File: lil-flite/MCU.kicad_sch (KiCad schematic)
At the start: 12 parts, among them SW401 PTS645SM70-2 LFS, SW402 PTS645SM70-2 LFS, U101 STM32F103C8T6, U401 W25Q128JVSIQ

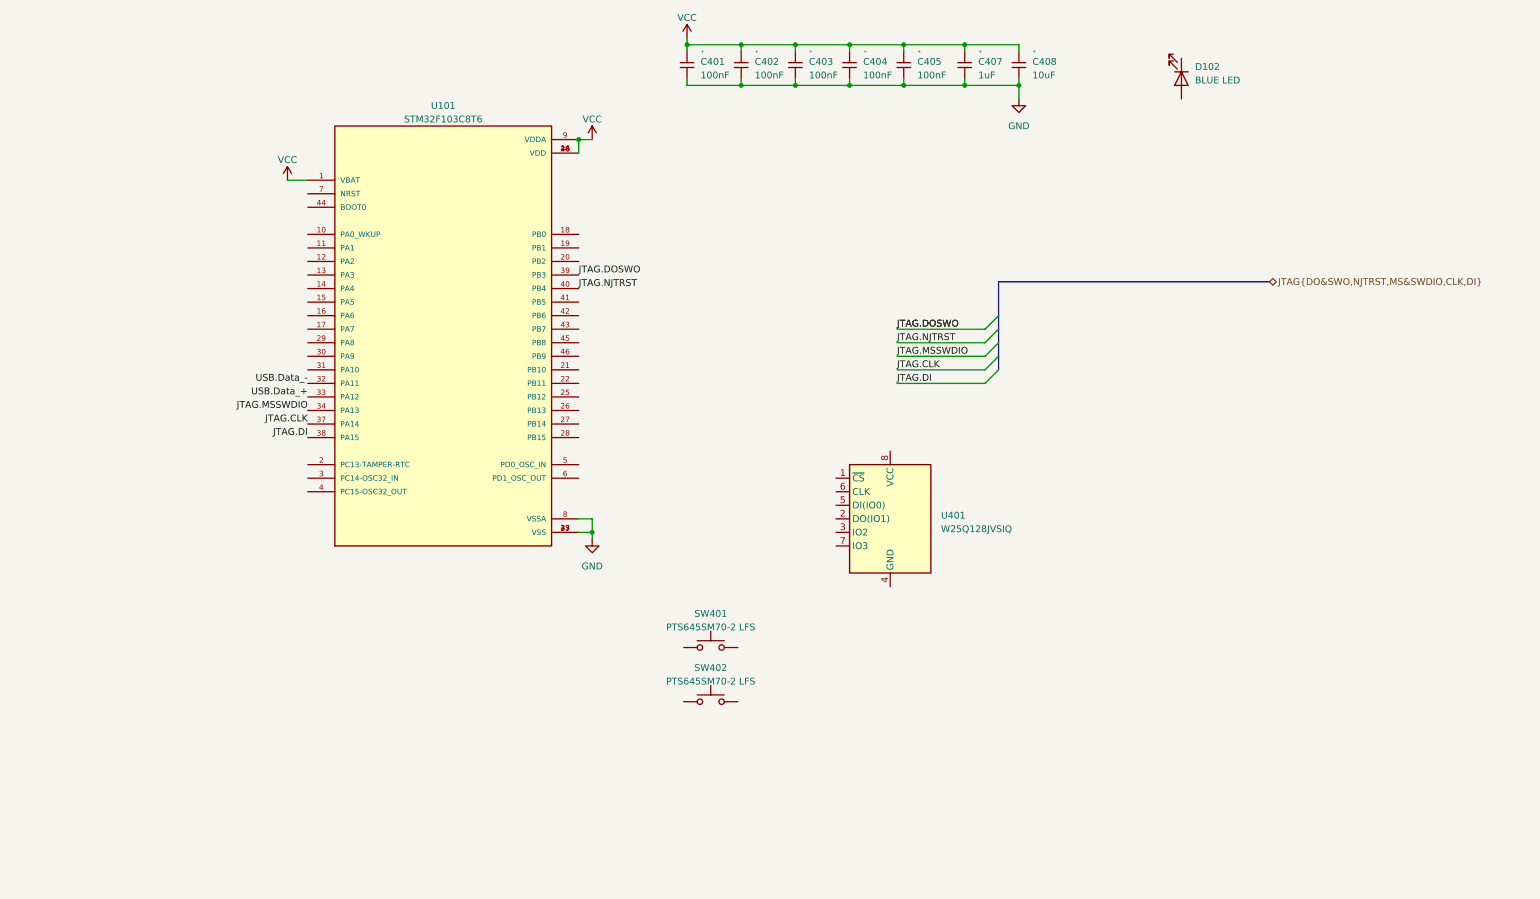
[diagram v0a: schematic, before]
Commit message: Almost finished
Need to double check everything
routing done
more vias maybe
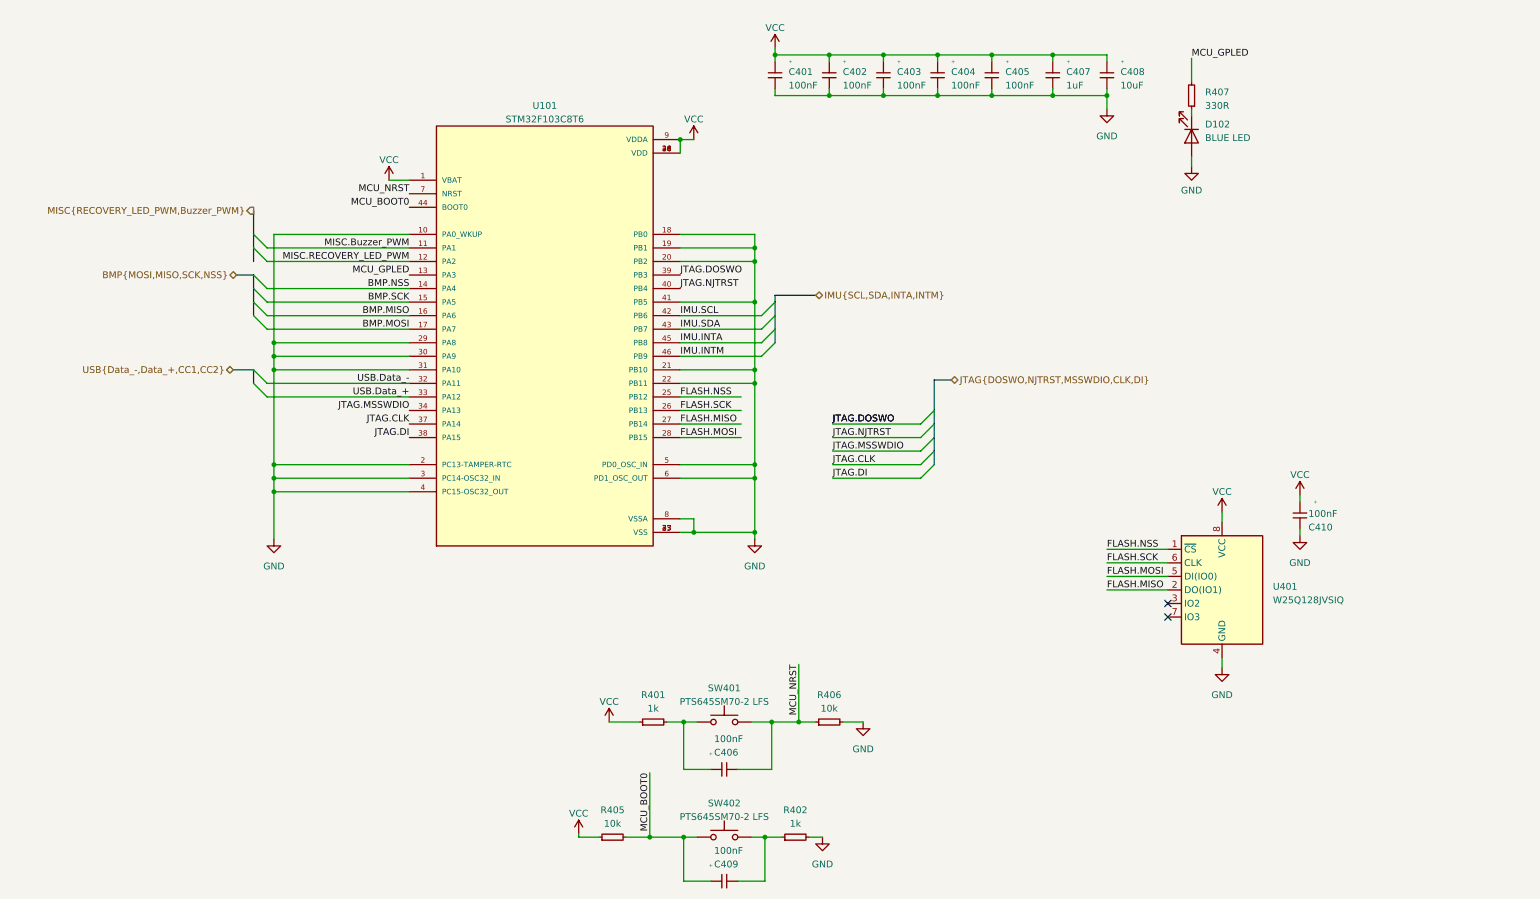
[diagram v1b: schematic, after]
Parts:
- added C406, C409, C410: 100nF, Capacitor_SMD:C_0603_1608Metric_Pad1.08x0.95mm_HandSolder, symbol PCM_Generic-50:C,IEC
- added R401, R402: 1k, Resistor_SMD:R_0603_1608Metric_Pad0.98x0.95mm_HandSolder, symbol PCM_Generic-50:R,IEC
- added R405, R406: 10k, Resistor_SMD:R_0603_1608Metric_Pad0.98x0.95mm_HandSolder, symbol PCM_Generic-50:R,IEC
- added R407: 330R, Resistor_SMD:R_0603_1608Metric_Pad0.98x0.95mm_HandSolder, symbol PCM_Generic-50:R,IEC
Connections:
- net GND: now also D102.2 (A), U101.10 (PA0_WKUP), U101.18 (PB0), U101.19 (PB1), U101.2 (PC13-TAMPER-RTC), U101.20 (PB2), U101.21 (PB10), U101.22 (PB11), U101.29 (PA8), U101.3 (PC14-OSC32_IN), U101.30 (PA9), U101.31 (PA10), U101.4 (PC15-OSC32_OUT), U101.41 (PB5), U101.5 (PD0_OSC_IN), U101.6 (PD1_OSC_OUT), U401.4 (GND), C410.1 (+), R402.2 (-), R406.2 (-)
- net VCC: now also U401.8 (VCC), C410.2 (-), R401.1 (+), R405.1 (+)
- net MCU_BOOT0: now reaches SW402.1, SW402.3
- net MCU_BOOT0: now also U101.44 (BOOT0), C409.2 (-), R405.2 (-)
- net at SW402.2, SW402.4: now also C409.1 (+), R402.1 (+)
- net at D102.1 (K): now also R407.1 (+)
- net at SW401.1, SW401.3: now also C406.2 (-), R401.2 (-)
- net MCU_NRST: now reaches SW401.2, SW401.4
- net MCU_NRST: now also U101.7 (NRST), C406.1 (+), R406.1 (+)
- net FLASH.NSS: now reaches U401.1 (~{CS})
- net FLASH.NSS: now also U101.25 (PB12)
- net FLASH.MISO: now reaches U401.2 (DO(IO1))
- net FLASH.MISO: now also U101.27 (PB14)
- net FLASH.MOSI: now reaches U401.5 (DI(IO0))
- net FLASH.MOSI: now also U101.28 (PB15)
- net FLASH.SCK: now reaches U401.6 (CLK)
- net FLASH.SCK: now also U101.26 (PB13)
- net MISC.Buzzer_PWM: now reaches U101.11 (PA1)
- net MISC.RECOVERY_LED_PWM: now reaches U101.12 (PA2)
- net MCU_GPLED: now reaches U101.13 (PA3)
- net MCU_GPLED: now also R407.2 (-)
- net BMP.NSS: now reaches U101.14 (PA4)
- net BMP.SCK: now reaches U101.15 (PA5)
- net BMP.MISO: now reaches U101.16 (PA6)
- net BMP.MOSI: now reaches U101.17 (PA7)
- net IMU.SCL: now reaches U101.42 (PB6)
- net IMU.SDA: now reaches U101.43 (PB7)
- net IMU.INTA: now reaches U101.45 (PB8)
- net IMU.INTM: now reaches U101.46 (PB9)
- no-connect marks 0 -> 2
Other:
- moved on the sheet: C401, C402, C403, C404, C405, C407, C408, D102, SW401, SW402, U101, U401
